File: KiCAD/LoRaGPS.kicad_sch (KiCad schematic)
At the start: 23 parts, among them J1 GPS, J2 battery 9V, U3 M78AR05-0.5, U4 24FC256, U5 BNO055, U7 BME280

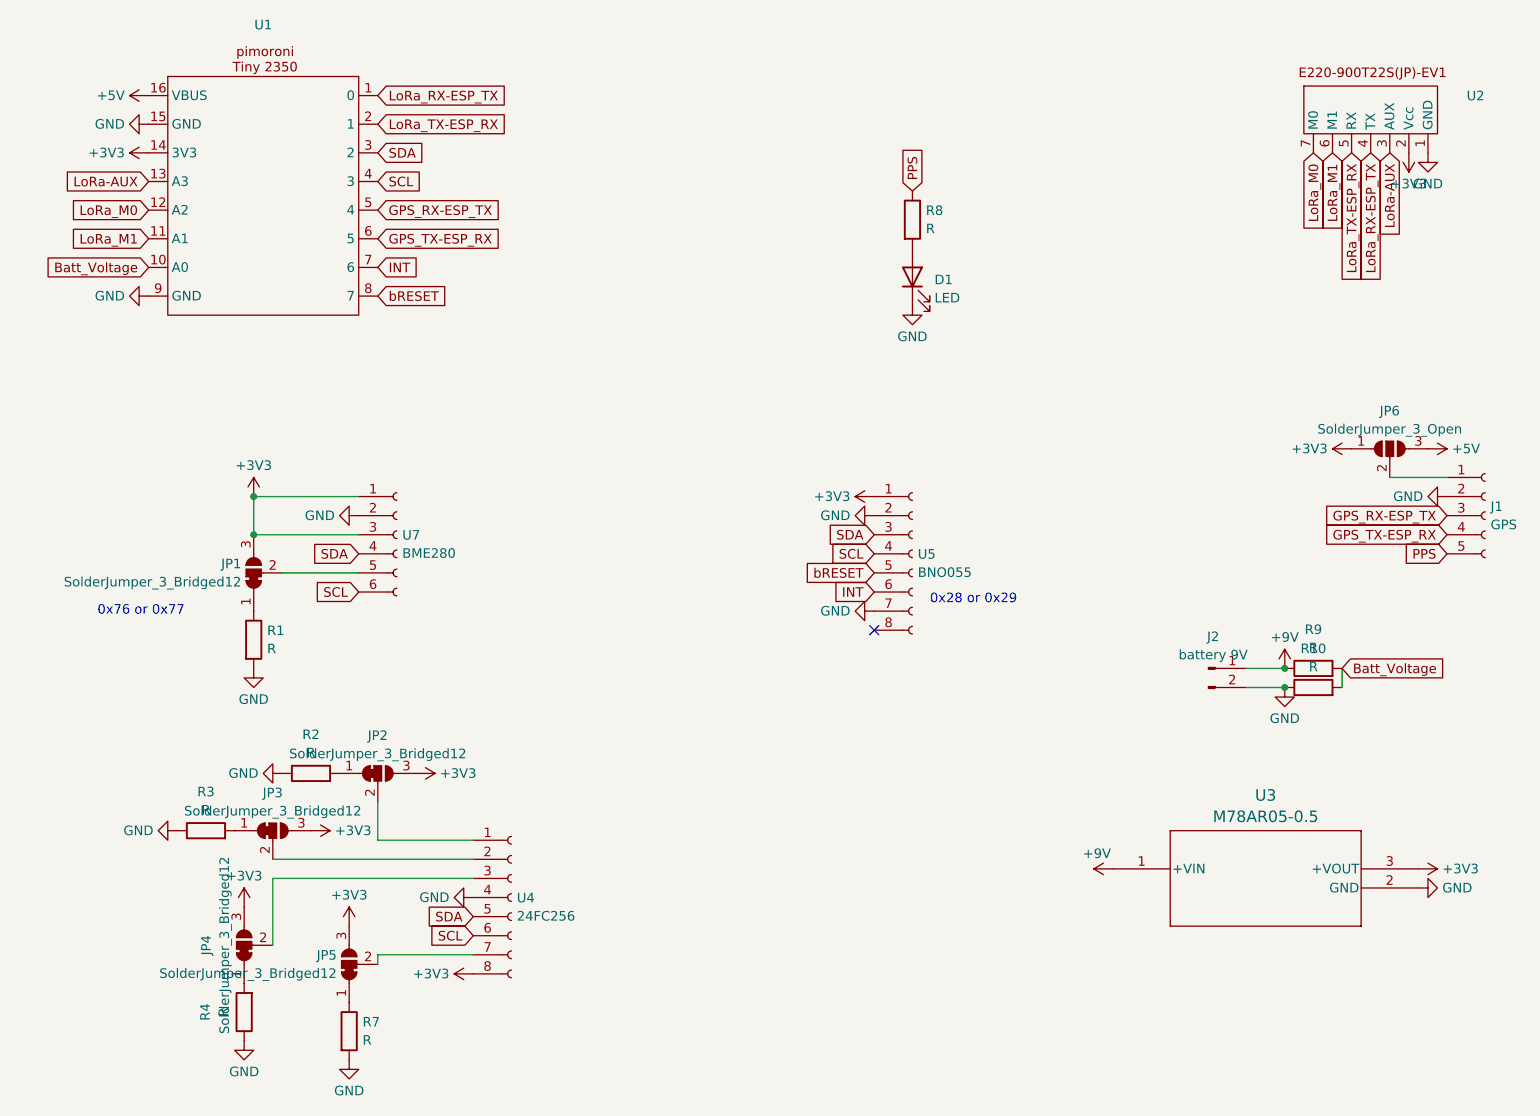
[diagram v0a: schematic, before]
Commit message: add reference on schematic
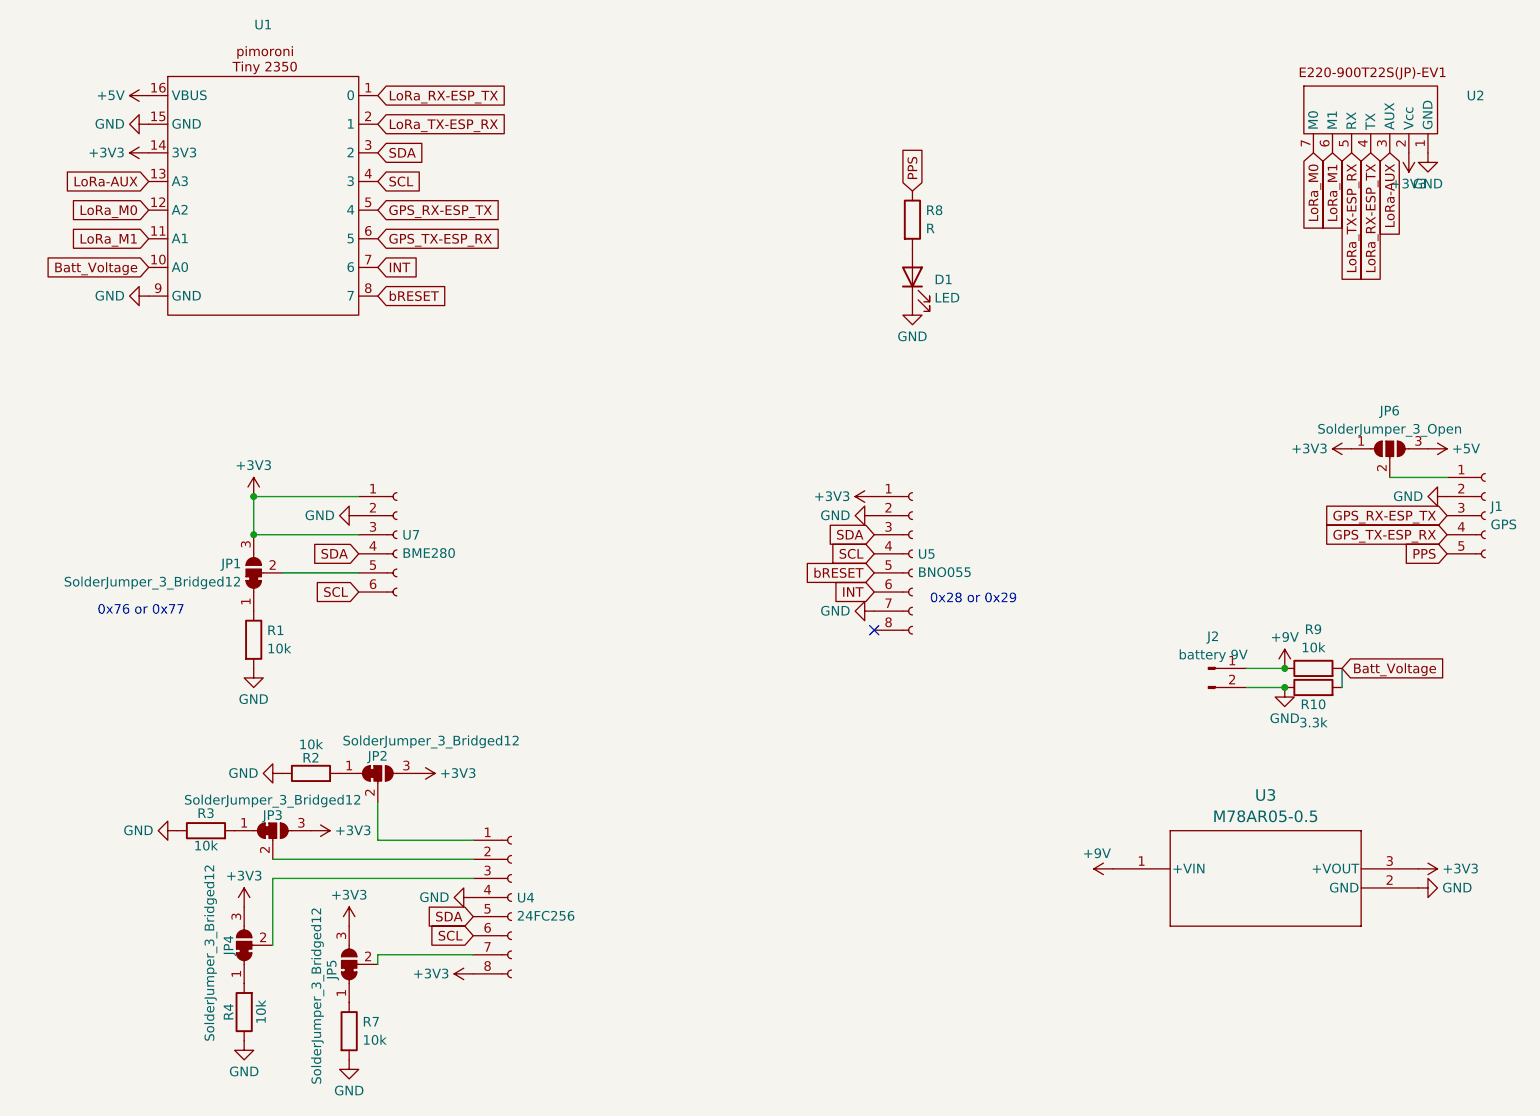
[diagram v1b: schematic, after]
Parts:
- R1, R2, R3, R4, R7, R9: value R -> 10k
- R10: value R -> 3.3k
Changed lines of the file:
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@@
 		(on_board yes)
 		(dnp no)
-		(fields_autoplaced yes)
 		(property "Reference" "JP3"
-			(at 73.66 143.5565 0)
+			(at 73.66 146.558 0)
 			(effects
 				(font
@@
 		)
 		(property "Value" "SolderJumper_3_Bridged12"
-			(at 73.66 145.9808 0)
+			(at 73.66 144.526 0)
 			(effects
 				(font
@@
 		(on_board yes)
 		(dnp no)
-		(fields_autoplaced yes)
 		(property "Reference" "R10"
-			(at 212.09 124.3795 90)
-			(effects
-				(font
-					(size 1.27 1.27)
-				)
-			)
-		)
-		(property "Value" "R"
-			(at 212.09 126.8038 90)
+			(at 212.09 131.826 90)
+			(effects
+				(font
+					(size 1.27 1.27)
+				)
+			)
+		)
+		(property "Value" "3.3k"
+			(at 212.09 134.2503 90)
 			(effects
 				(font
@@
 		(on_board yes)
 		(dnp no)
-		(fields_autoplaced yes)
 		(property "Reference" "R4"
-			(at 64.6895 172.72 90)
-			(effects
-				(font
-					(size 1.27 1.27)
-				)
-			)
-		)
-		(property "Value" "R"
-			(at 67.1138 172.72 90)
+			(at 67.818 172.72 90)
+			(effects
+				(font
+					(size 1.27 1.27)
+				)
+			)
+		)
+		(property "Value" "10k"
+			(at 72.136 172.72 90)
 			(effects
 				(font
@@
 			)
 		)
-		(property "Value" "R"
+		(property "Value" "10k"
 			(at 72.898 124.4021 0)
 			(effects
@@
 		(on_board yes)
 		(dnp no)
-		(fields_autoplaced yes)
 		(property "Reference" "R2"
-			(at 78.74 135.8095 90)
-			(effects
-				(font
-					(size 1.27 1.27)
-				)
-			)
-		)
-		(property "Value" "R"
-			(at 78.74 138.2338 90)
+			(at 78.74 138.938 90)
+			(effects
+				(font
+					(size 1.27 1.27)
+				)
+			)
+		)
+		(property "Value" "10k"
+			(at 78.74 137.16 90)
 			(effects
 				(font
@@
 		(on_board yes)
 		(dnp no)
-		(fields_autoplaced yes)
 		(property "Reference" "JP5"
-			(at 82.1691 165.1578 90)
+			(at 81.534 168.402 0)
 			(effects
 				(font
@@
 		)
 		(property "Value" "SolderJumper_3_Bridged12"
-			(at 82.1691 167.5821 90)
+			(at 79.502 182.372 0)
 			(effects
 				(font
@@
 			)
 		)
-		(property "Value" "R"
+		(property "Value" "10k"
 			(at 212.09 124.2638 90)
 			(effects
@@
 		(on_board yes)
 		(dnp no)
-		(fields_autoplaced yes)
 		(property "Reference" "JP2"
-			(at 87.63 135.9365 0)
+			(at 87.63 138.684 0)
 			(effects
 				(font
@@
 		)
 		(property "Value" "SolderJumper_3_Bridged12"
-			(at 87.63 138.3608 0)
+			(at 94.742 136.652 0)
 			(effects
 				(font
@@
 		(dnp no)
 		(property "Reference" "JP4"
-			(at 64.8165 163.83 0)
+			(at 67.818 163.83 0)
 			(effects
 				(font
@@
 		)
 		(property "Value" "SolderJumper_3_Bridged12"
-			(at 67.2408 163.83 0)
+			(at 65.278 164.846 0)
 			(effects
 				(font
@@
 		(on_board yes)
 		(dnp no)
-		(fields_autoplaced yes)
 		(property "Reference" "R3"
-			(at 64.77 143.4295 90)
-			(effects
-				(font
-					(size 1.27 1.27)
-				)
-			)
-		)
-		(property "Value" "R"
-			(at 64.77 145.8538 90)
+			(at 64.77 146.304 90)
+			(effects
+				(font
+					(size 1.27 1.27)
+				)
+			)
+		)
+		(property "Value" "10k"
+			(at 64.77 150.622 90)
 			(effects
 				(font
@@
 			)
 		)
-		(property "Value" "R"
+		(property "Value" "10k"
 			(at 85.598 176.4721 0)
 			(effects
